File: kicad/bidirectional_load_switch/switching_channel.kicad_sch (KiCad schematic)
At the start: 14 parts, among them U201 SN74LVC1G17DCKR, U202 UCC23313DWYR, U203 SISS94DN-T1-GE3, U204 SISS94DN-T1-GE3

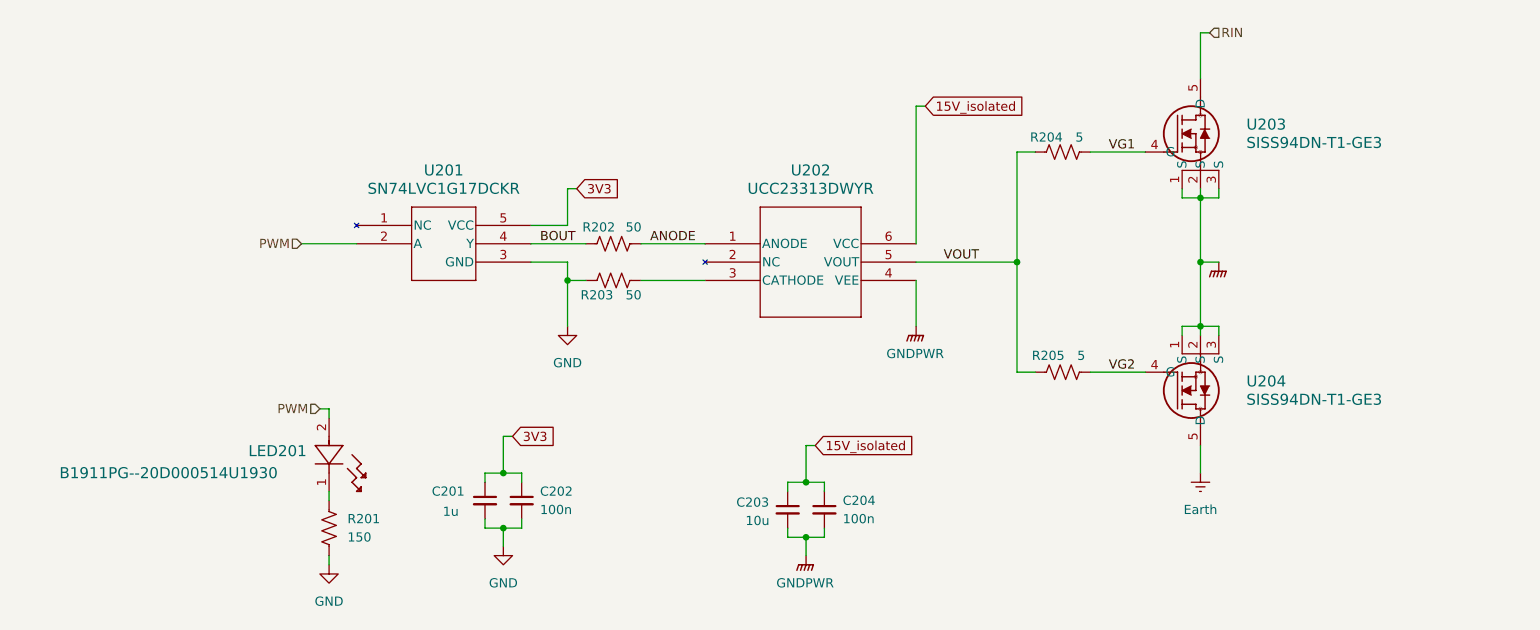
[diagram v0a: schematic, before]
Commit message: i hate layouts
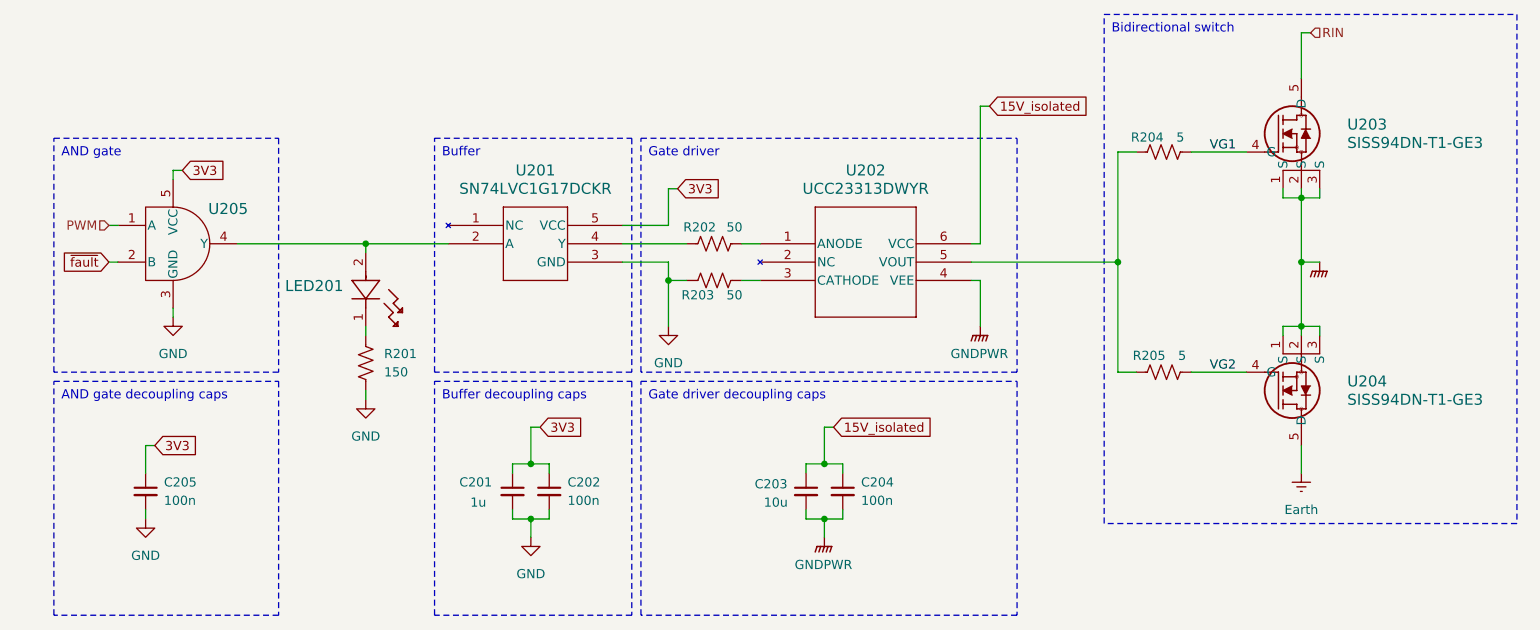
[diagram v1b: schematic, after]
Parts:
- added C205: 100n, Capacitor_SMD:C_0603_1608Metric, symbol Device:C_Small
- added U205: SN74LVC1G08DCKR, and_gate_SN74LVC1G08DCKR:DCK5, symbol and_gate_SN74LVC1G08DCKR:SN74LVC1G08DCKR
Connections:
- net 3V3: now also C205.1, U205.5 (VCC)
- net GND: now also C205.2, U205.3 (GND)
- net PWM: now also U205.1 (A); no longer LED201.2, U201.2 (A)
- net ANODE: no longer names the net of R202.2, U202.1 (ANODE)
- net BOUT: no longer names the net of R202.1, U201.4 (Y)
- net VOUT: no longer names the net of R204.1, R205.1, U202.5 (VOUT)
- new net: LED201.2, U201.2 (A), U205.4 (Y)
- new net ~{fault}: U205.2 (B)
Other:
- company: (none) -> University of Wisconsin-Platteville
- moved on the sheet: C201, C202, C203, C204, LED201, R201, R202, R203, R204, R205, U201, U202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
